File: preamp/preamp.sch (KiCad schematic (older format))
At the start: 32 parts, among them P1 CONNECTOR, P2 CONNECTOR, P3 CONNECTOR, P4 CONNECTOR, P5 CONNECTOR, U1 LM741, U2 LM741, U3 LM741

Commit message: 
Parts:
- removed P1: CONNECTOR, symbol CONNECTOR
- added P1: Plug entrada, symbol CONN_2
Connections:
- wire segments 75 -> 76
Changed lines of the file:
@@
-EESchema Schematic File Version 2  date sáb 07 jul 2012 02:10:25 ART
+EESchema Schematic File Version 2  date sáb 07 jul 2012 14:32:06 ART
 LIBS:power
 LIBS:device
@@
 Comment4 ""
 $EndDescr
+$Comp
+L GND #PWR01
+U 1 1 4FF86E92
+P 1750 1550
+F 0 "#PWR01" H 1750 1550 30  0001 C CNN
+F 1 "GND" H 1750 1480 30  0001 C CNN
+	1    1750 1550
+	1    0    0    -1
+$EndComp
 Wire Wire Line
 	2150 600  1950 600
@@
 Connection ~ 5500 6400
 Wire Wire Line
-	6300 6400 5500 6400
-Wire Wire Line
-	1500 800  1950 800
+	5500 6400 6300 6400
+Wire Wire Line
+	1950 800  1500 800
 Connection ~ 3850 800
 Wire Wire Line
@@
 Wire Wire Line
 	2850 4950 2850 4600
-Wire Wire Line
-	1500 800  1500 1050
 Wire Wire Line
 	6800 1150 7000 1150
@@
 Connection ~ 6300 1700
 Wire Wire Line
-	6300 2200 6300 2400
-Wire Wire Line
-	2950 2200 2950 2400
+	6300 2400 6300 2200
+Wire Wire Line
+	2950 2400 2950 2200
 Wire Wire Line
 	4850 950  4700 950
@@
 	6700 3850 6650 3850
 Wire Wire Line
-	6650 3850 6650 3000
+	6650 3000 6650 3850
 Connection ~ 5500 4500
 Wire Wire Line
@@
 Connection ~ 4600 4000
 Wire Wire Line
-	4600 4000 4000 4000
+	4000 4000 4600 4000
 Wire Wire Line
 	4000 4000 4000 4200
@@
 Connection ~ 2850 4000
 Wire Wire Line
-	2850 4000 2250 4000
+	2250 4000 2850 4000
 Wire Wire Line
 	2250 4000 2250 4100
@@
 	5800 800  3850 800
 Wire Wire Line
-	5500 6400 5500 5300
-Wire Wire Line
-	2950 2400 6300 2400
+	5500 5300 5500 6400
+Wire Wire Line
+	6300 2400 2950 2400
 Wire Wire Line
 	2700 600  2550 600
+Wire Wire Line
+	1500 800  1500 1350
+Wire Wire Line
+	1500 1350 1750 1350
+$Comp
+L CONN_2 P1
+U 1 1 4FF86010
+P 2100 1450
+F 0 "P1" V 2050 1450 40  0000 C CNN
+F 1 "Plug entrada" V 2150 1450 40  0000 C CNN
+	1    2100 1450
+	1    0    0    -1
+$EndComp
 $Comp
 L C C8
@@
 $EndComp
 $Comp
-L PWR_FLAG #FLG2
+L PWR_FLAG #FLG02
 U 1 1 4FF4DBC4
 P 6800 1150
-F 0 "#FLG2" H 6800 1245 30  0001 C CNN
+F 0 "#FLG02" H 6800 1245 30  0001 C CNN
 F 1 "PWR_FLAG" H 6800 1330 30  0000 C CNN
 	1    6800 1150
@@
 $EndComp
 $Comp
-L PWR_FLAG #FLG1
+L PWR_FLAG #FLG03
 U 1 1 4FF4DBBF
 P 6800 800
-F 0 "#FLG1" H 6800 895 30  0001 C CNN
+F 0 "#FLG03" H 6800 895 30  0001 C CNN
 F 1 "PWR_FLAG" H 6800 980 30  0000 C CNN
 	1    6800 800
@@
 $EndComp
 $Comp
-L PWR_FLAG #FLG3
+L PWR_FLAG #FLG04
 U 1 1 4FF4DBB2
 P 8250 950
-F 0 "#FLG3" H 8250 1045 30  0001 C CNN
+F 0 "#FLG04" H 8250 1045 30  0001 C CNN
 F 1 "PWR_FLAG" H 8250 1130 30  0000 C CNN
 	1    8250 950
@@
 $EndComp
 $Comp
-L GND #PWR3
+L GND #PWR05
 U 1 1 4FF4DBA0
 P 8250 950
-F 0 "#PWR3" H 8250 950 30  0001 C CNN
+F 0 "#PWR05" H 8250 950 30  0001 C CNN
 F 1 "GND" H 8250 880 30  0001 C CNN
 	1    8250 950
@@
 	1    0    0    -1
 $EndComp
-$Comp
-L CONNECTOR P1
-U 1 1 4FEE38E3
-P 1500 1050
-F 0 "P1" H 1850 1150 70  0000 C CNN
-F 1 "CONNECTOR" H 1850 950 70  0000 C CNN
-	1    1500 1050
-	1    0    0    -1
-$EndComp
 Text Label 2400 5750 0    60   ~ 0
 1
@@
 1
 $Comp
-L GND #PWR1
+L GND #PWR06
 U 1 1 4FEE3676
 P 5100 2500
-F 0 "#PWR1" H 5100 2500 30  0001 C CNN
+F 0 "#PWR06" H 5100 2500 30  0001 C CNN
 F 1 "GND" H 5100 2430 30  0001 C CNN
 	1    5100 2500
@@
 $EndComp
 $Comp
-L GND #PWR2
+L GND #PWR07
 U 1 1 4FEE2F30
 P 6300 6550
-F 0 "#PWR2" H 6300 6550 30  0001 C CNN
+F 0 "#PWR07" H 6300 6550 30  0001 C CNN
 F 1 "GND" H 6300 6480 30  0001 C CNN
 	1    6300 6550

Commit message: empeze el pcb del pre
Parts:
- removed U1, U2, U3: LM741, symbol LM741
- added C10, C11, C12, C9: C, symbol C
- added R1, R6: R, symbol R
- added U1, U2: N35532, symbol N35532
- renumbered P2 to 20+1, P3 to 20-1
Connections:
- wire segments 76 -> 81
- no-connect marks 6 -> 0
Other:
- moved on the sheet: 20+1, 20-1, P4, R7

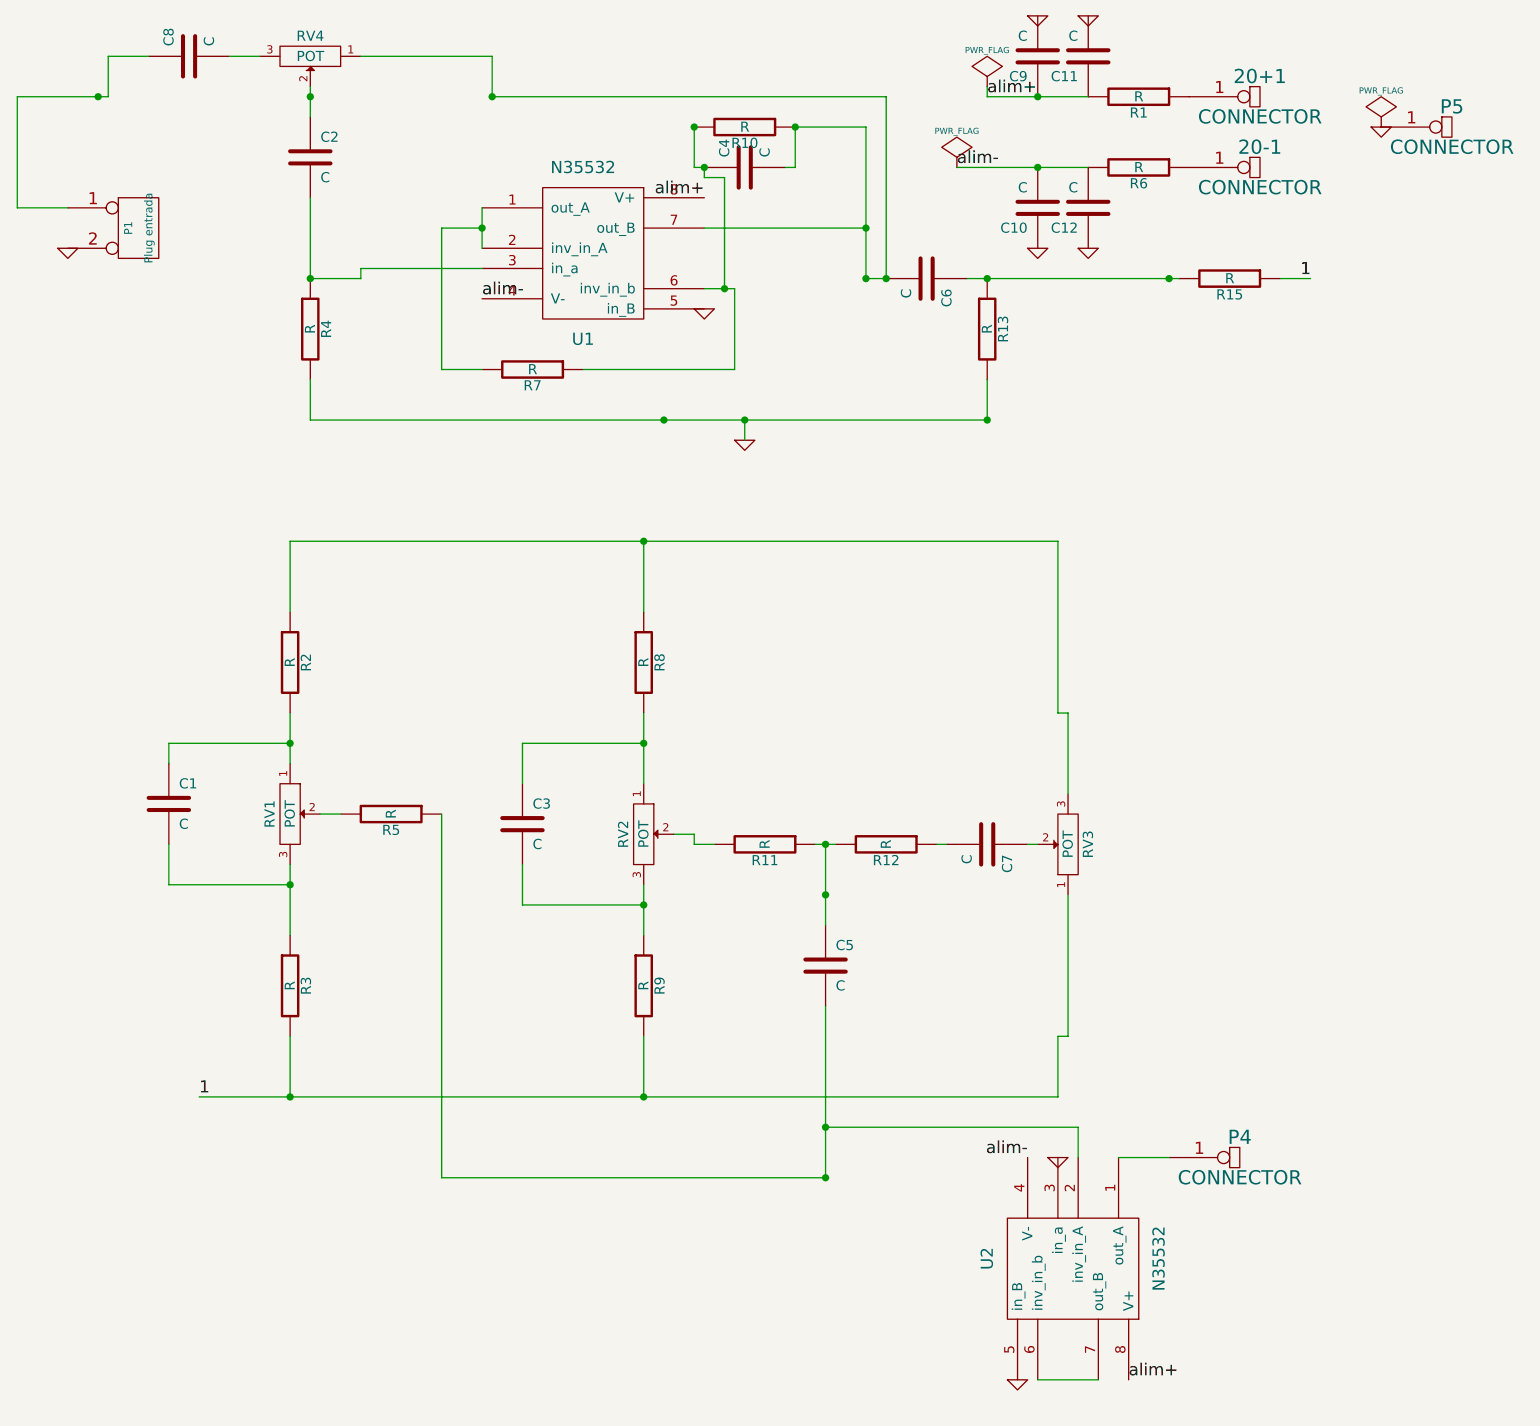
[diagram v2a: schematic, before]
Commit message: pre conectado
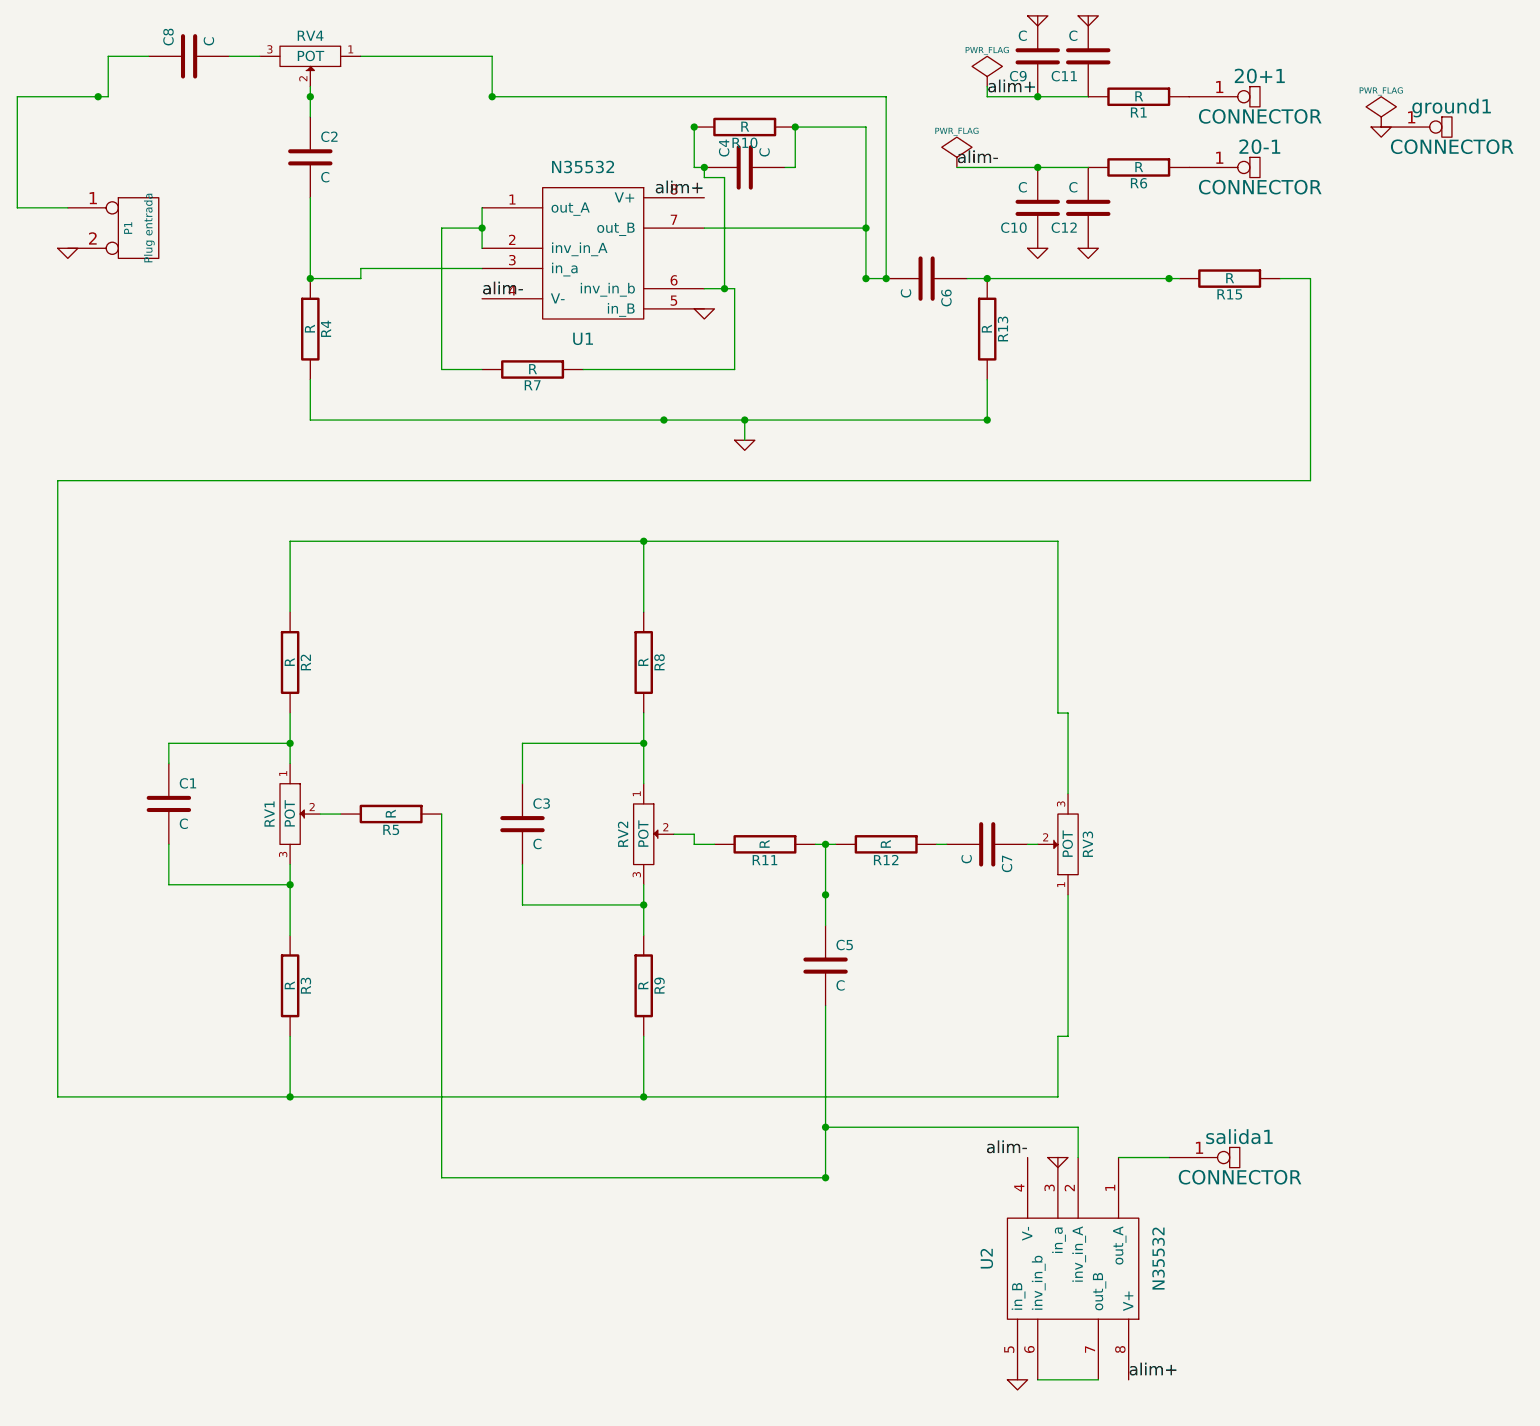
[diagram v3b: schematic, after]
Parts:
- renumbered P5 to ground1, P4 to salida1
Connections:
- net 1: no longer names the net of R15.1, R3.2, R9.2, RV3.1
